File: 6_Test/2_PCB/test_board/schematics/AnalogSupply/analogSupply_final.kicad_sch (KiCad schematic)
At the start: 17 parts

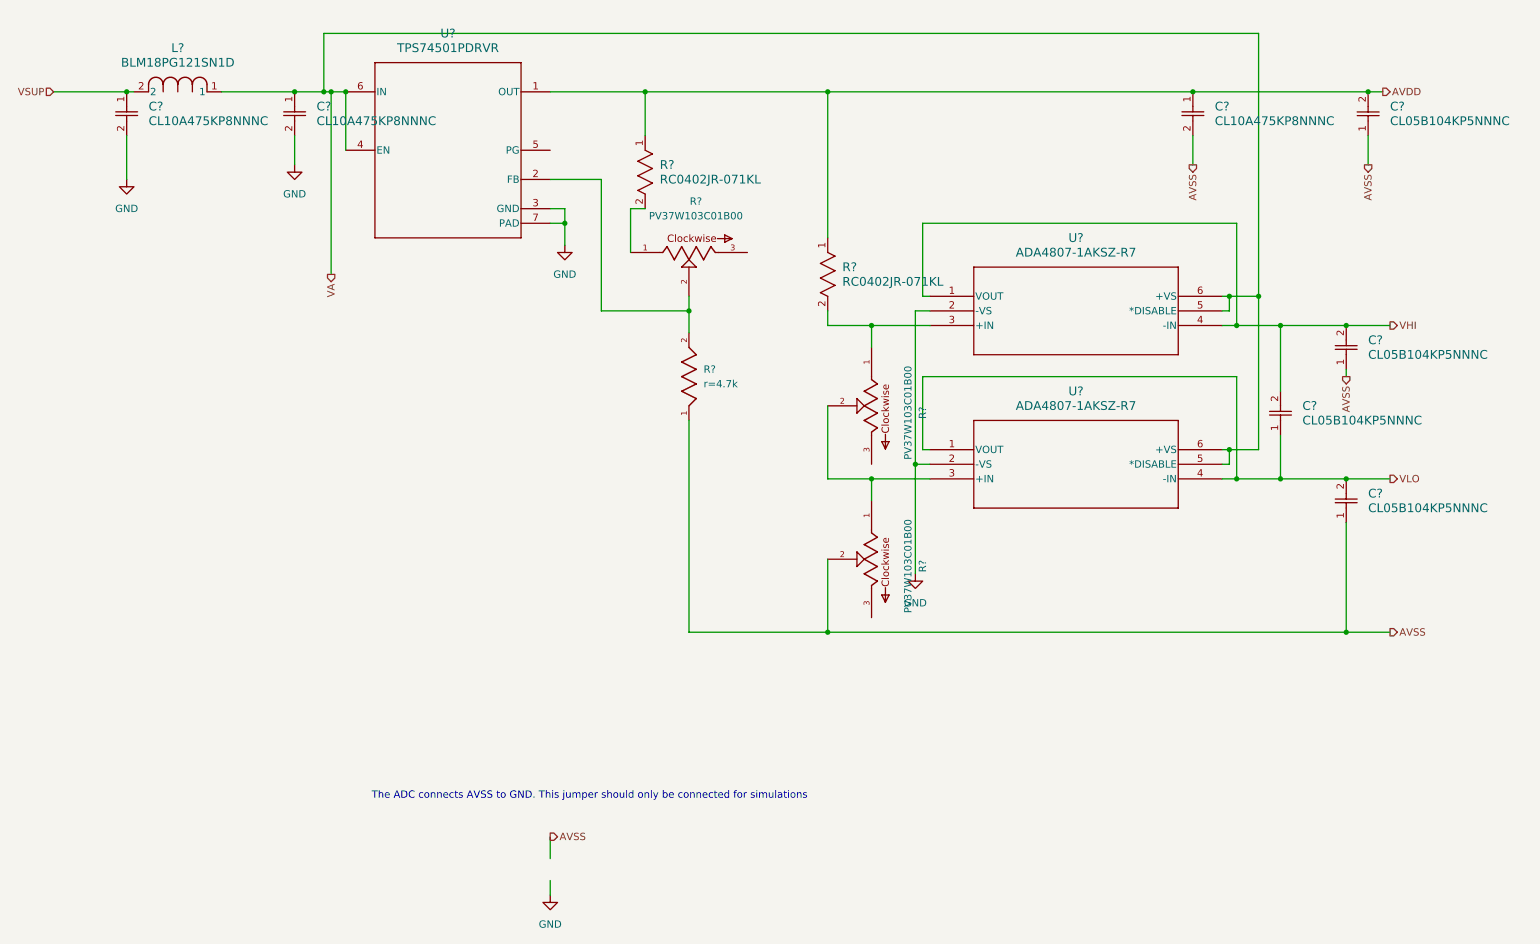
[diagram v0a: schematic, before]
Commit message: Corrections to schematic 11_20_24
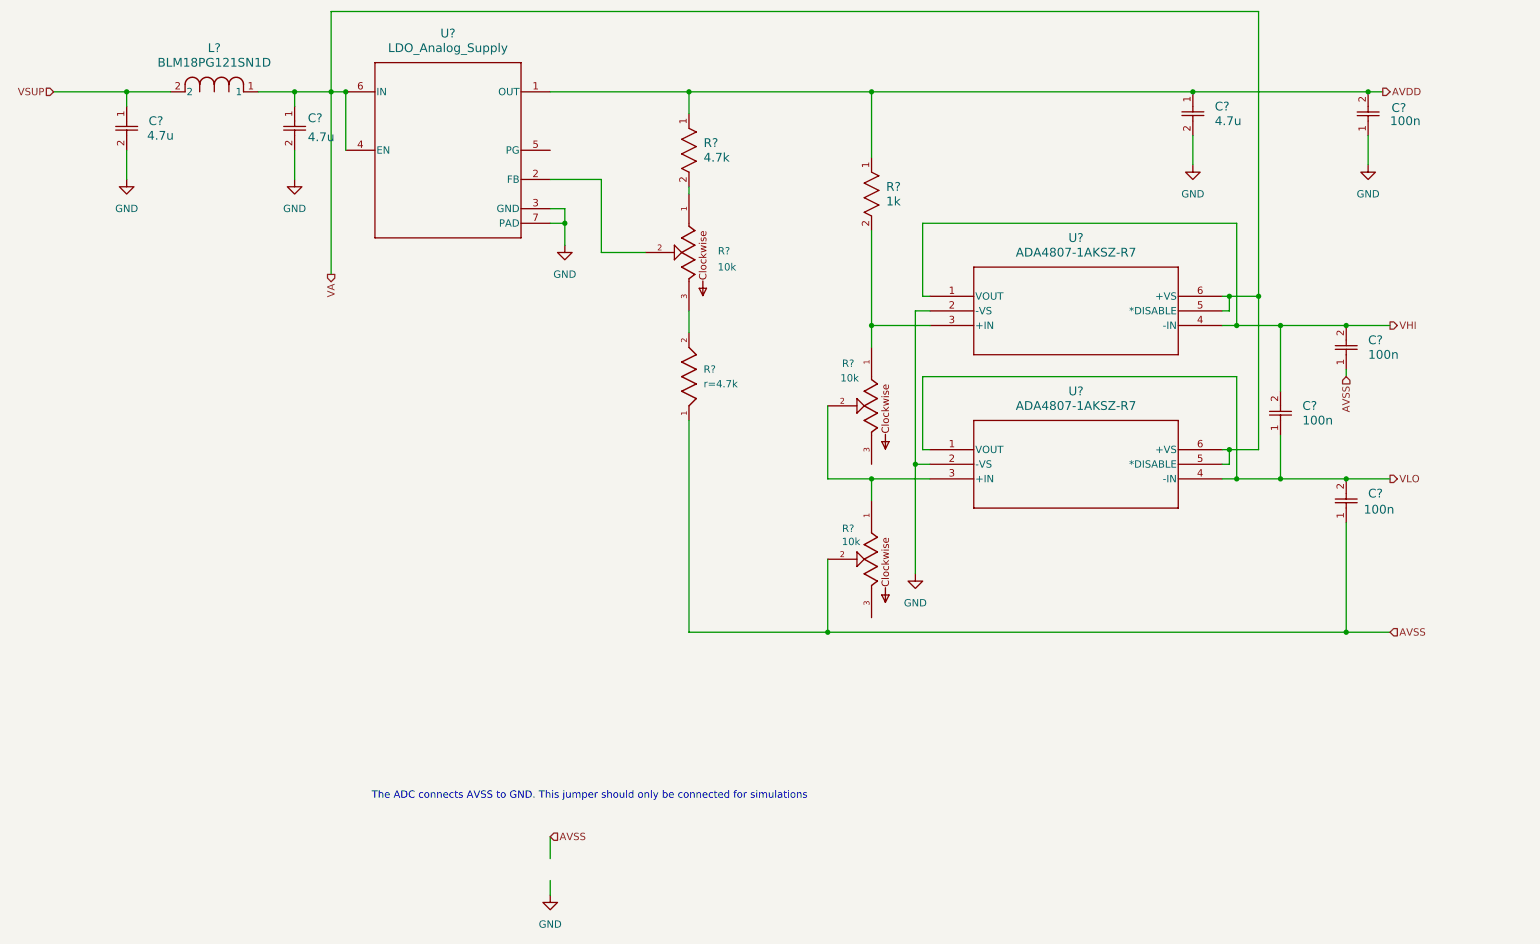
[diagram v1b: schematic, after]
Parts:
- C? (x4): value CL05B104KP5NNNC -> 100n
- C? (x3): value CL10A475KP8NNNC -> 4.7u
- R?: value RC0402JR-071KL -> 1k
- R?: value RC0402JR-071KL -> 4.7k
- R? (x3): value PV37W103C01B00 -> 10k
- U? (x2): footprint KS-6_ADI -> opampADA4807Footprints:KS-6_ADI
- U?: value TPS74501PDRVR -> LDO_Analog_Supply
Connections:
- net AVSS: no longer C?.1, C?.2
- net GND: now also C?.1, C?.2
- net at R?.2, U?.2 (FB): no longer R?.2
- net at R?.3: now also R?.2
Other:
- moved on the sheet: C?, L?, R?
